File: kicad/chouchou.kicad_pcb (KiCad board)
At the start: 2 copper layers, 206.6 x 122 mm, 21 parts

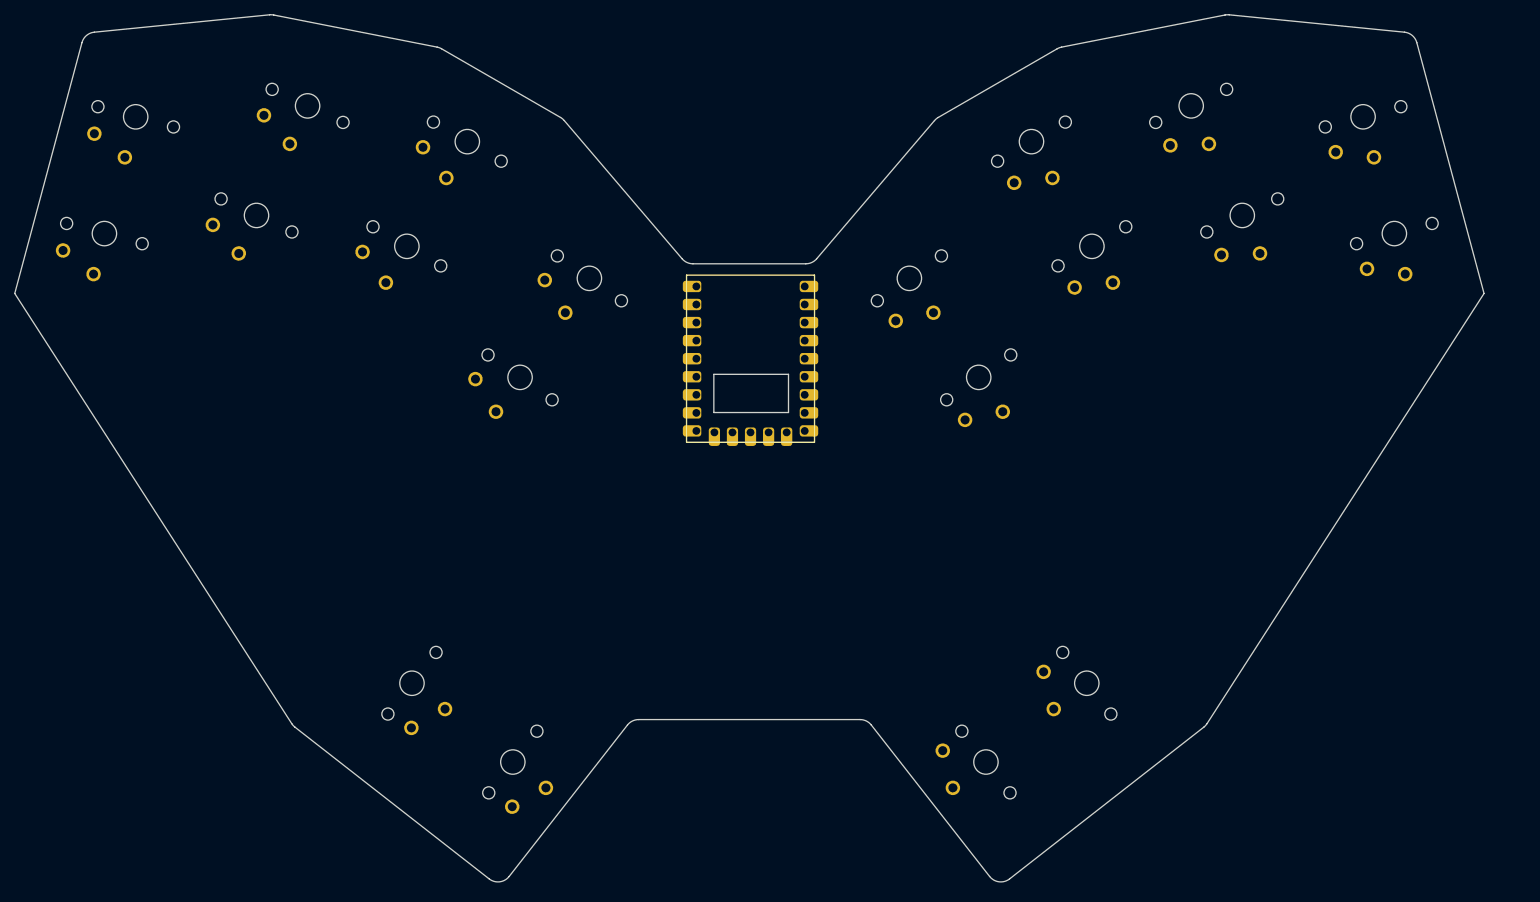
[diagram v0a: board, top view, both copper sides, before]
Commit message: add wiring
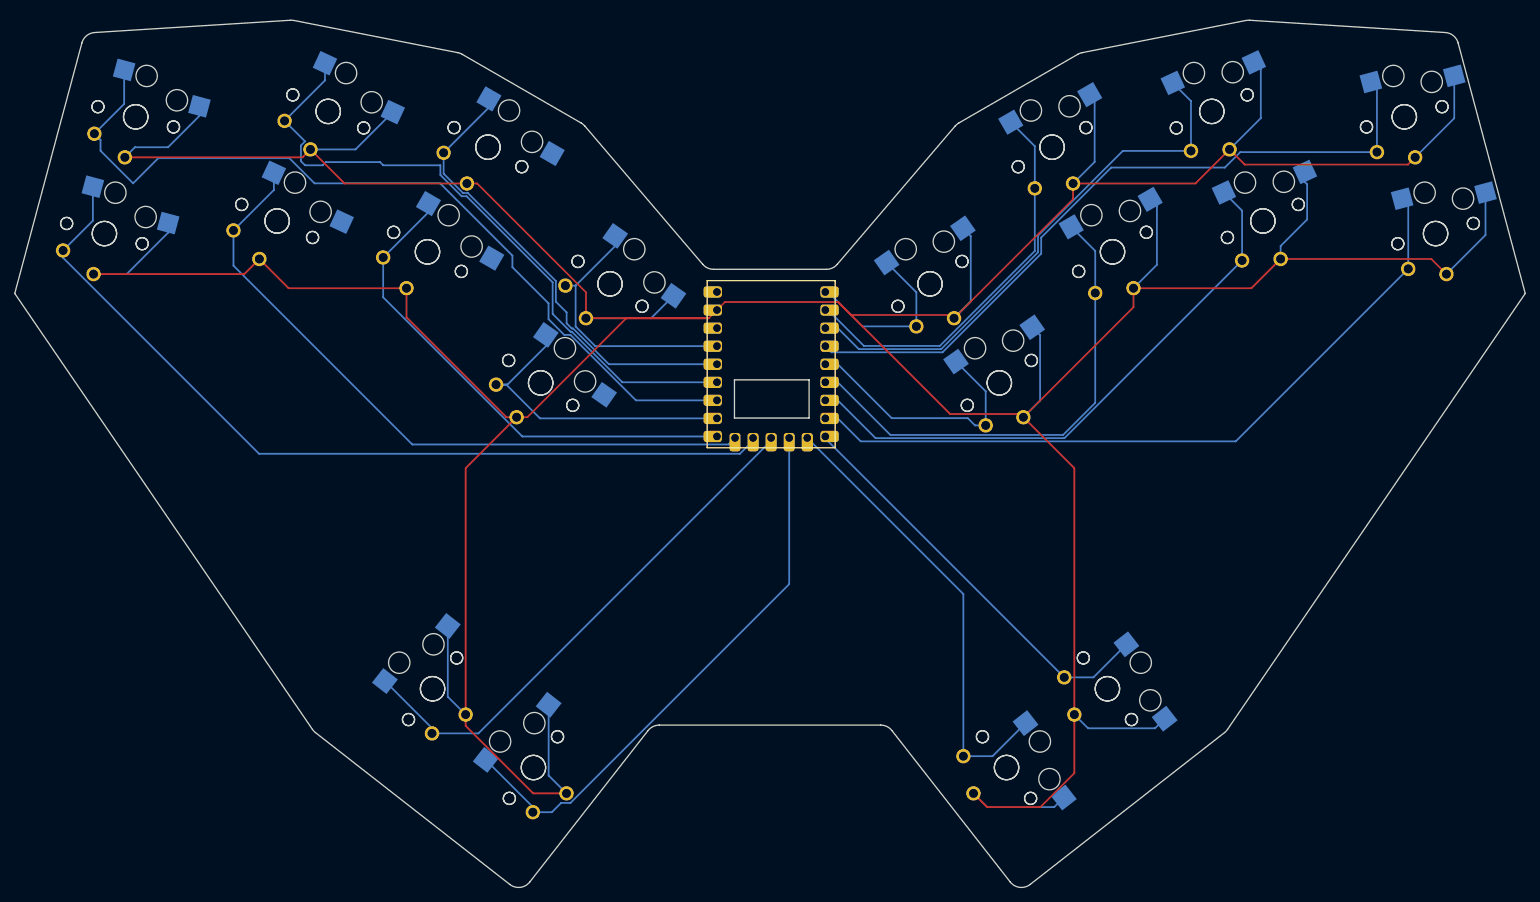
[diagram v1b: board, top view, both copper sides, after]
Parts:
- added S21: , PG1350, F.Cu at (36.6, 136.6)
- added S22: , PG1350, F.Cu at (41.0, 120.2)
- added S23: , PG1350, F.Cu at (60.9, 134.8)
- added S24: , PG1350, F.Cu at (68.1, 119.4)
- added S25: , PG1350, F.Cu at (82.0, 139.2)
- added S26: , PG1350, F.Cu at (90.5, 124.4)
- added S27: , PG1350, F.Cu at (98.0, 157.6)
- added S28: , PG1350, F.Cu at (107.7, 143.7)
- added S29: , PG1350, F.Cu at (82.8, 200.6)
- added S30: , PG1350, F.Cu at (96.9, 211.7)
- added S31: , PG1350, F.Cu at (223.8, 136.6)
- added S32: , PG1350, F.Cu at (219.4, 120.2)
- added S33: , PG1350, F.Cu at (199.5, 134.8)
- added S34: , PG1350, F.Cu at (192.3, 119.4)
- added S35: , PG1350, F.Cu at (178.4, 139.2)
- added S36: , PG1350, F.Cu at (169.9, 124.4)
- added S37: , PG1350, F.Cu at (162.5, 157.6)
- added S38: , PG1350, F.Cu at (152.7, 143.7)
- added S39: , PG1350, F.Cu at (177.7, 200.6)
- added S40: , PG1350, F.Cu at (163.5, 211.7)
- moved S12 5.80 mm to (219.4, 120.2), turned to 15 degrees
- moved S11 5.80 mm to (223.8, 136.6), turned to 15 degrees
- moved S6 3.00 mm to (90.5, 124.4), turned to -30 degrees
- moved S19 3.00 mm to (177.7, 200.6), turned to -52 degrees
- moved S5 3.00 mm to (82.0, 139.2), turned to -30 degrees
- moved S17 3.00 mm to (162.5, 157.6), turned to 35 degrees
- moved S3 3.00 mm to (60.9, 134.8), turned to -25 degrees
- moved S10 3.00 mm to (96.9, 211.7), turned to 52 degrees
- moved S7 3.00 mm to (98.0, 157.6), turned to -35 degrees
- moved S13 3.00 mm to (199.5, 134.8), turned to 25 degrees
- moved S9 3.00 mm to (82.8, 200.6), turned to 52 degrees
- moved S16 3.00 mm to (169.9, 124.4), turned to 30 degrees
- moved S20 3.00 mm to (163.5, 211.7), turned to -52 degrees
- moved S15 3.00 mm to (178.4, 139.2), turned to 30 degrees
- moved S18 3.00 mm to (152.7, 143.7), turned to 35 degrees
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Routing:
- net GND: track 0.00 -> 774.7 mm
- net GP12: track 0.00 -> 121.3 mm
- net GP26: track 0.00 -> 119.9 mm
- net GP7: track 0.00 -> 103.6 mm
- net GP3: track 0.00 -> 101.1 mm
- net GP13: track 0.00 -> 96.7 mm
- net GP27: track 0.00 -> 92.7 mm
- net GP6: track 0.00 -> 81.8 mm
- net GP10: track 0.00 -> 80.0 mm
- net GP2: track 0.00 -> 76.2 mm
- net GP11: track 0.00 -> 75.2 mm
- net GP14: track 0.00 -> 70.9 mm
- net GP5: track 0.00 -> 69.0 mm
- net GP28: track 0.00 -> 65.3 mm
- net GP9: track 0.00 -> 64.5 mm
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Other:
- board size 206.6 x 122 mm -> 212.4 x 122 mm
- net class Default removed

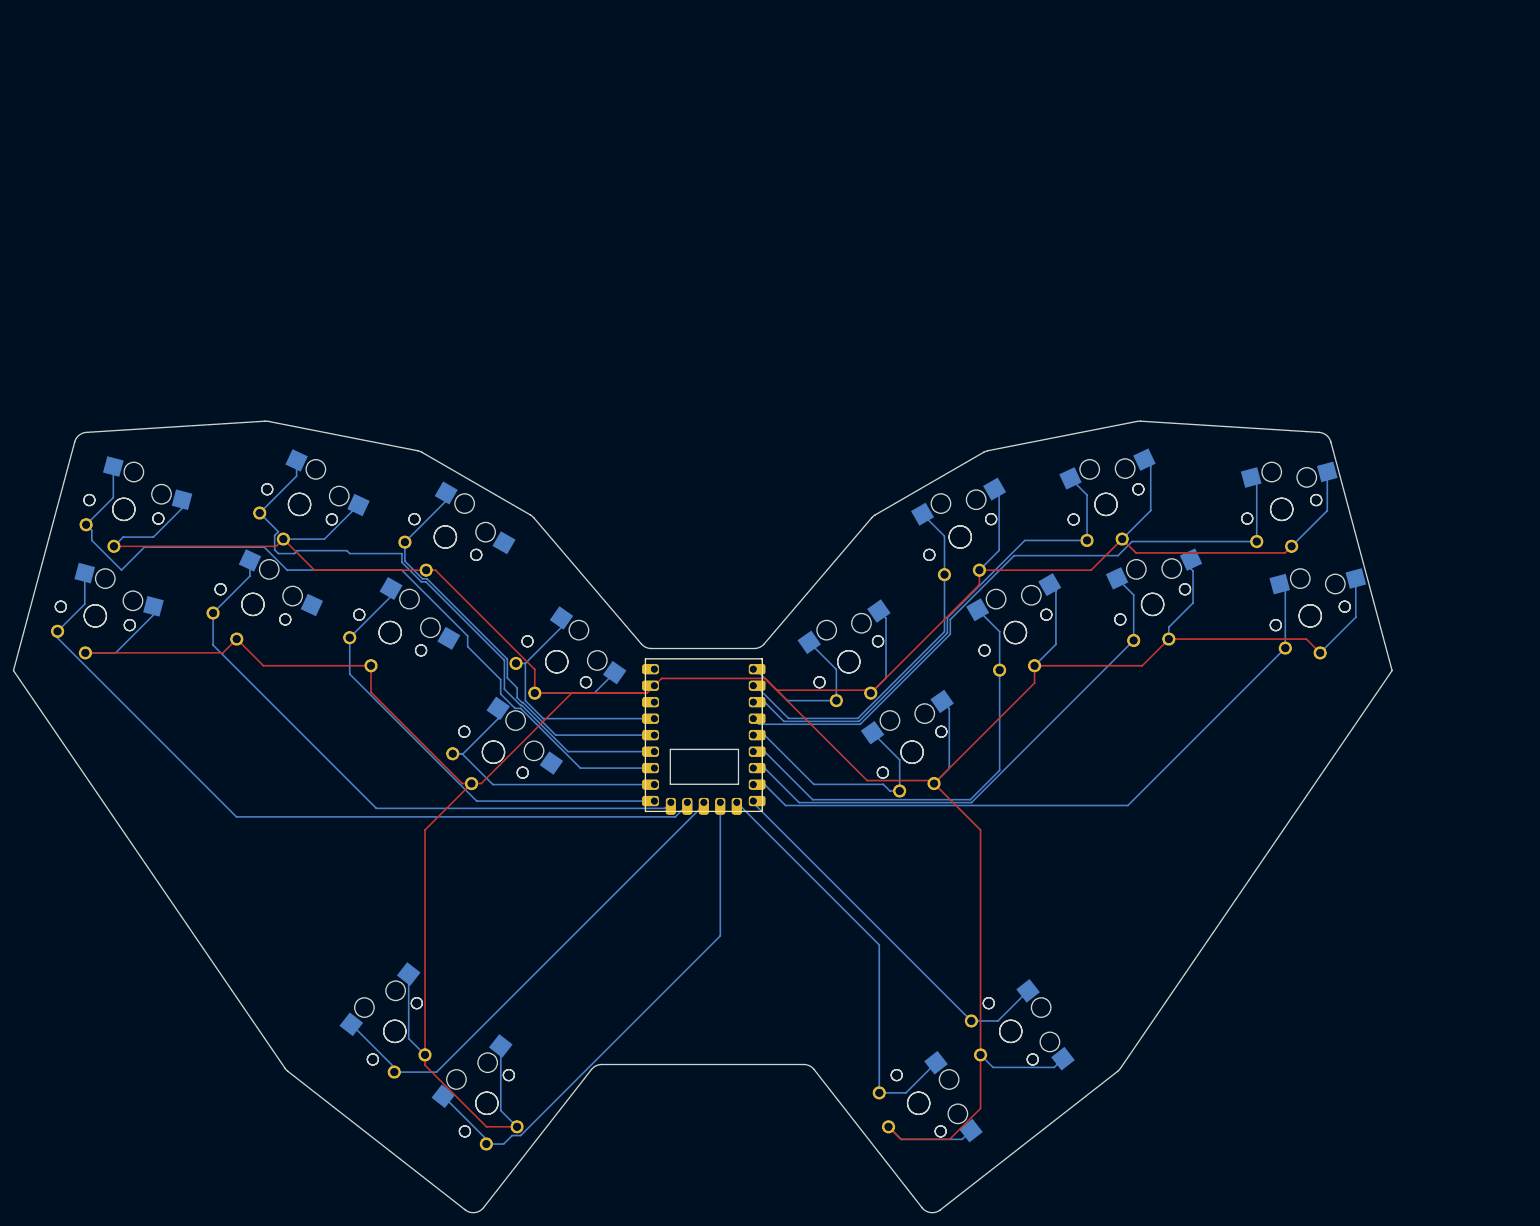
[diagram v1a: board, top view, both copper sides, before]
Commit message: Update design
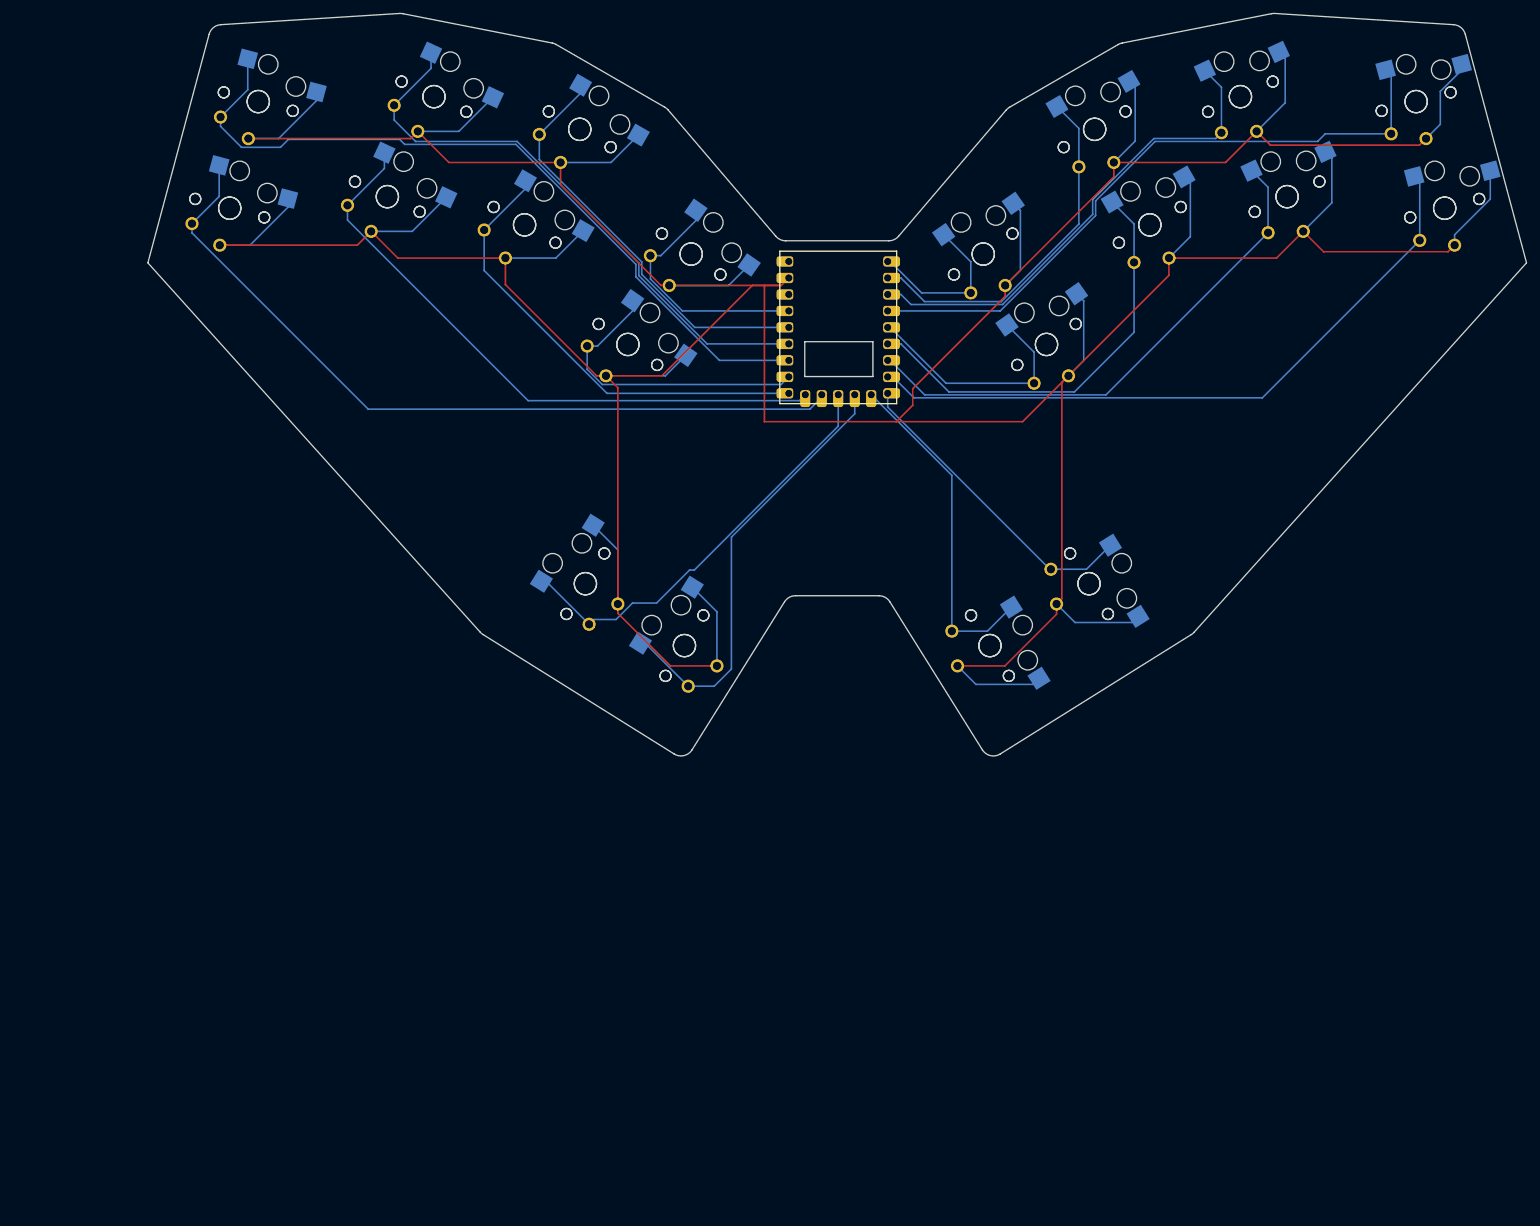
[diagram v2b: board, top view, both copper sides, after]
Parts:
- moved S10 76.8 mm to (127.4, 141.2), turned to 58 degrees
- moved S30 76.8 mm to (127.4, 141.2), turned to -122 degrees
- moved S29 75.0 mm to (112.1, 131.6), turned to -122 degrees
- moved S9 75.0 mm to (112.1, 131.6), turned to 58 degrees
- moved S20 71.4 mm to (174.5, 141.2), turned to -58 degrees
- moved S40 71.4 mm to (174.5, 141.2), turned to 122 degrees
- moved S19 70.0 mm to (189.7, 131.6), turned to -58 degrees
- moved S39 70.0 mm to (189.7, 131.6), turned to 122 degrees
- moved RP2040Zero1 66.1 mm to (140.9, 104.9)
- moved S28 66.1 mm to (128.4, 80.9)
- moved S8 66.1 mm to (128.4, 80.9)
- moved S1 66.1 mm to (57.3, 73.8)
- moved S11 66.1 mm to (244.5, 73.8)
- moved S12 66.1 mm to (240.1, 57.4)
- moved S18 66.1 mm to (173.4, 80.9)
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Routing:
- net GND: track 774.7 -> 840.4 mm
- net GP9: track 64.5 -> 52.3 mm
- net GP10: track 80.0 -> 68.0 mm
- net GP8: track 58.5 -> 48.3 mm
- net GP11: track 75.2 -> 66.0 mm
- net GP27: track 92.7 -> 89.0 mm
- net GP26: track 119.9 -> 116.8 mm
- net GP15: track 43.9 -> 46.9 mm
- net GP5: track 69.0 -> 66.3 mm
- net GP13: track 96.7 -> 95.2 mm
- net GP2: track 76.2 -> 75.0 mm
- net GP1: track 56.6 -> 55.4 mm
- net GP28: track 65.3 -> 64.4 mm
- net GP3: track 101.1 -> 100.4 mm
- net GP4: track 37.3 -> 36.8 mm
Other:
- board size 212.4 x 122 mm -> 212.4 x 114.4 mm
